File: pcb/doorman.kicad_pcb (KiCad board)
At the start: 4 copper layers, 37 x 37.2 mm, 61 parts, among them J1 USB-C Connector, J2 Screw Terminals, J3 3V3 Test Pad, J4 Extension Board Connector, J5 Siedle BUS RX Test Pad, J6 BUS Test Pad, J7 BUS RX Test Pad, J8 TX Test Pad, J9 RX Test Pad, Q1 BC847BPN, Q2 BC817-40, Q3 BC817-40, Q4 BC817-40, Q5 BC807-40, Q6 BC807-40, SW1 Button, SW2 Button, U2 AP63203WU, U3 GAQY252G3S, U4 ESP32-S3-MINI-1

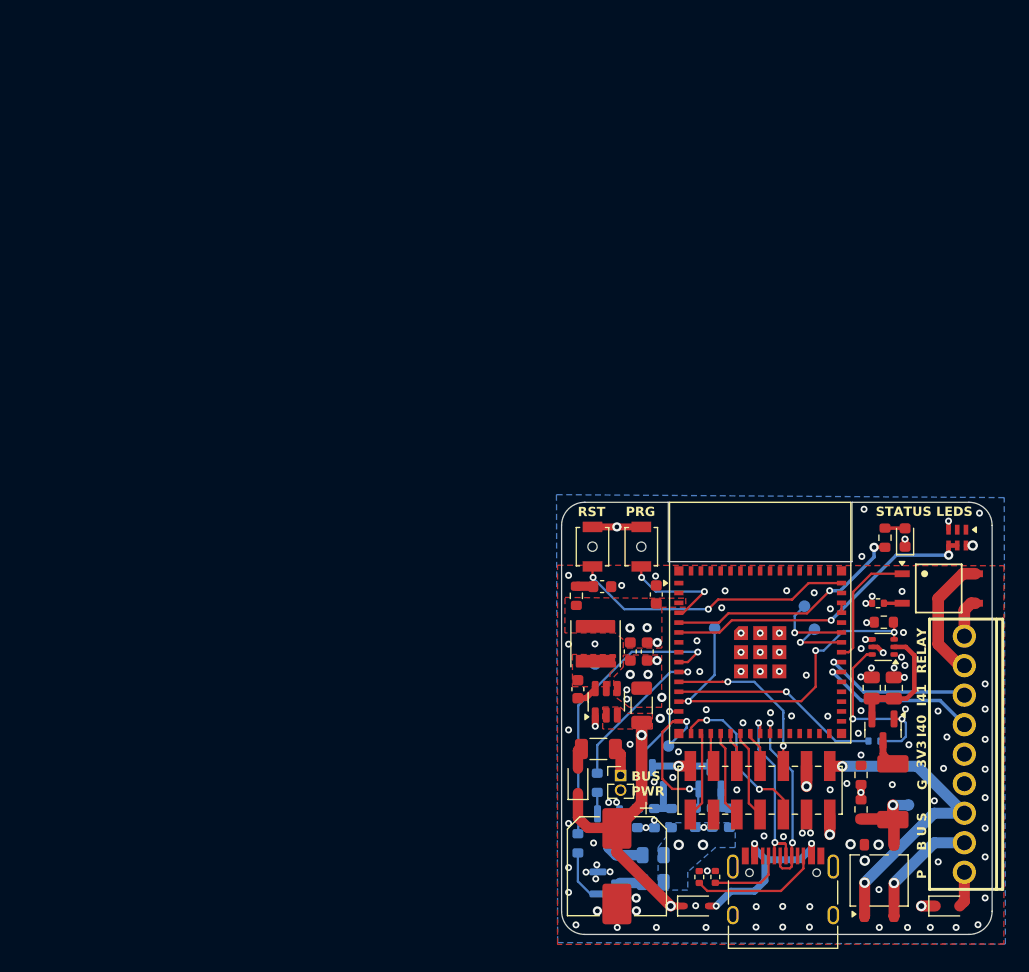
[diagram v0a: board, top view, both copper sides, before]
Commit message: WIP
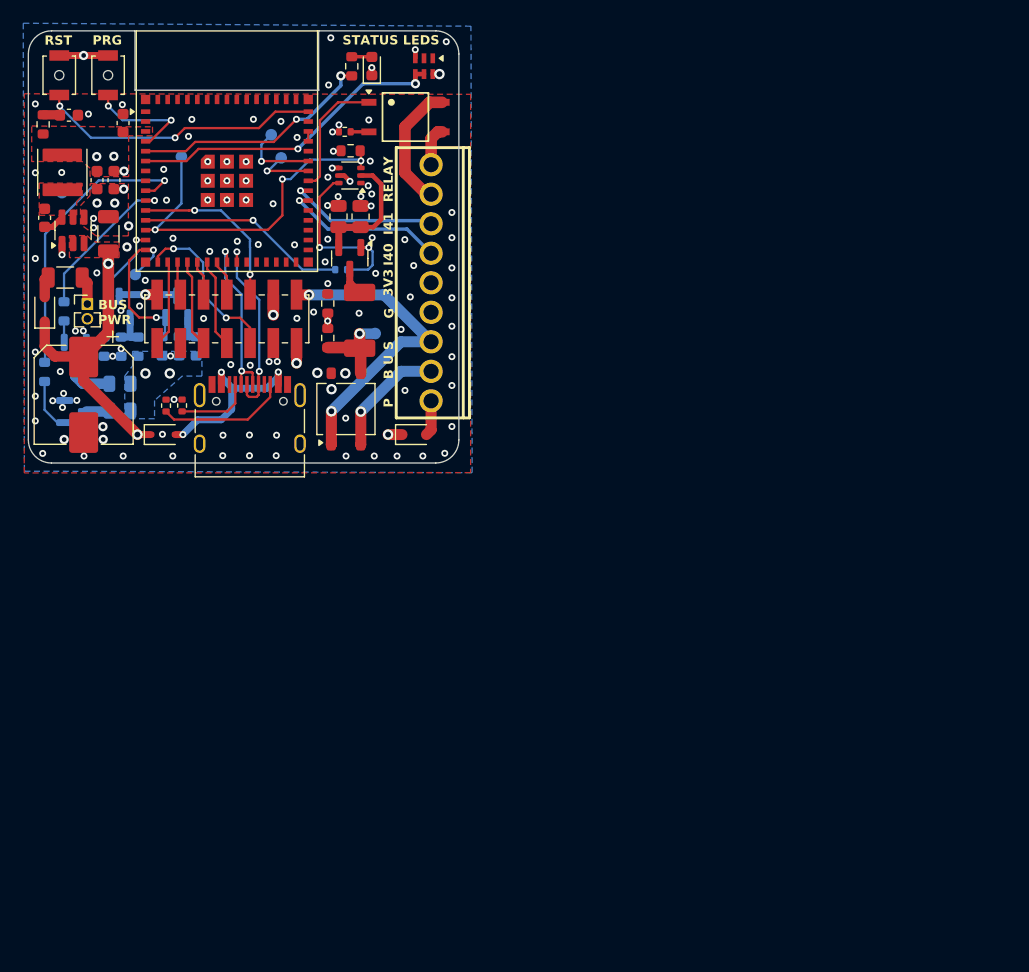
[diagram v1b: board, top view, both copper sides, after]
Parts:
- moved C1 61.3 mm to (84.4, 43.4)
- moved C6 61.3 mm to (88.3, 49.0)
- moved G*** 61.3 mm to (115.6, 44.4)
- moved J9 61.3 mm to (101.8, 45.0)
- moved R1 61.3 mm to (82.2, 44.2)
- moved R14 61.3 mm to (82.3, 65.5)
- moved R21 61.3 mm to (87.5, 63.3)
- moved R5 61.3 mm to (106.7, 62.5)
- moved C2 61.3 mm to (89.1, 44.0)
- moved C5 61.3 mm to (82.3, 52.2)
- moved C7 61.3 mm to (86.9, 49.0)
- moved D4 61.3 mm to (110.5, 39.1)
- moved D5 61.3 mm to (114.2, 70.9)
- moved D6 61.3 mm to (82.4, 60.1)
- moved J6 61.3 mm to (110.8, 62.2)
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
